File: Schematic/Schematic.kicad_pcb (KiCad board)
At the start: 2 copper layers, 67.5 x 55 mm, 17 parts, among them J3 FTDI, SW1 SW_Push, U1 ATmega328P-A, Y1 16 Mhz

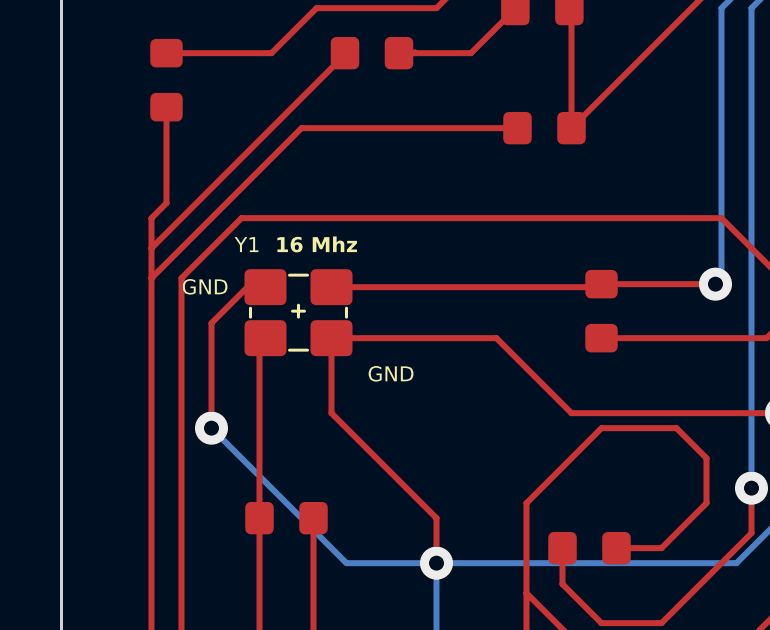
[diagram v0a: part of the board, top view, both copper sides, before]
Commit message: warnings still to do
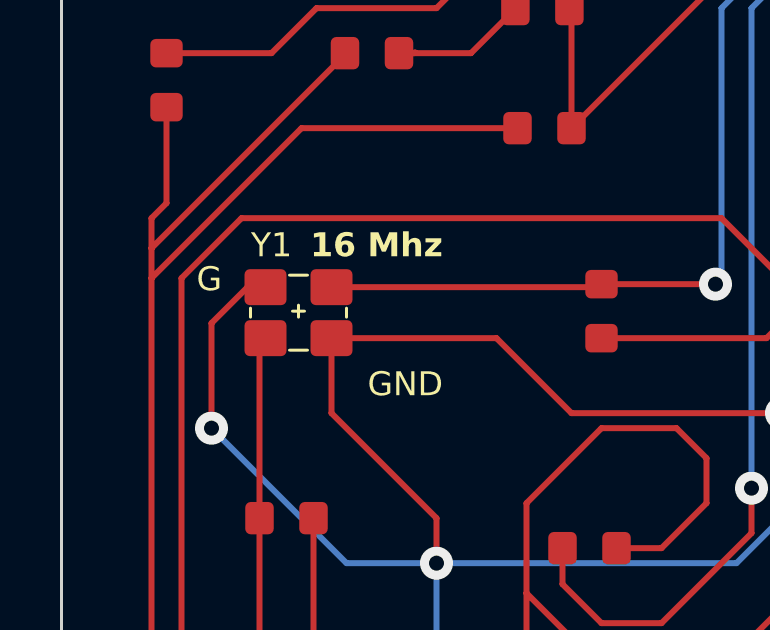
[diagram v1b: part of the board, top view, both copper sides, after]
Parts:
- C1, C2, C3, C4, C6, C7, D1, D2, R1, R2, R3: footprint Library:SMD_603 -> Library:SmD_603
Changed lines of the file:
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@@
 	(net 32 "A7")
 	(net 33 "A4")
-	(footprint "Library:SMD_603"
+	(footprint "Library:SmD_603"
 		(layer "F.Cu")
 		(at 146.6 122.5)
@@
 		(embedded_fonts no)
 	)
-	(footprint "Library:SMD_603"
+	(footprint "Library:SmD_603"
 		(layer "F.Cu")
 		(at 136.5 121.5)
@@
 			)
 		)
-		(property "Datasheet" "https://yageogroup.com/content/datasheet/asset/file/UPY-GPHC_X7R_6_3V-TO-250V"
+		(property "Datasheet" "https://yageogroup.com/content/datasheet/asset/file/PYU-RC_GROUP_51_ROHS_L"
 			(at 0 0 0)
 			(unlocked yes)
@@
 			(at -0.9 0)
 			(size 0.95 1.08)
-			(layers "F.Cu" "F.Paste")
+			(layers "F.Cu")
 			(roundrect_rratio 0.1968503937)
 			(net 3 "Net-(U1-XTAL1{slash}PB6)")
@@
 			(at 0.9 0)
 			(size 0.95 1.08)
-			(layers "F.Cu" "F.Paste")
+			(layers "F.Cu")
 			(roundrect_rratio 0.1968503937)
 			(net 2 "Net-(#PWR8-Pad1)")
@@
 		(embedded_fonts no)
 	)
-	(footprint "Library:SMD_603"
+	(footprint "Library:SmD_603"
 		(layer "F.Cu")
 		(at 145.1 108.5 180)
@@
 			)
 		)
-		(property "Datasheet" "https://yageogroup.com/content/datasheet/asset/file/UPY-GPHC_X7R_6_3V-TO-250V"
+		(property "Datasheet" "https://yageogroup.com/content/datasheet/asset/file/PYU-RC_GROUP_51_ROHS_L"
 			(at 0 0 180)
 			(unlocked yes)
@@
 			(at -0.9 0 180)
 			(size 0.95 1.08)
-			(layers "F.Cu" "F.Paste")
+			(layers "F.Cu")
 			(roundrect_rratio 0.1968503937)
 			(net 6 "RAW")
@@
 			(at 0.9 0 180)
 			(size 0.95 1.08)
-			(layers "F.Cu" "F.Paste")
+			(layers "F.Cu")
 			(roundrect_rratio 0.1968503937)
 			(net 17 "GND")
 			(pintype "passive")
+			(teardrops
+				(best_length_ratio 0.5)
+				(max_length 1)
+				(best_width_ratio 1)
+				(max_width 2)
+				(curved_edges no)
+				(filter_ratio 0.9)
+				(enabled yes)
+				(allow_two_segments yes)
+				(prefer_zone_connections yes)
+			)
 		)
 		(embedded_fonts no)
@@
 		(embedded_fonts no)
 	)
-	(footprint "Library:SMD_603"
+	(footprint "Library:SmD_603"
 		(layer "F.Cu")
 		(at 168.5 116.6 -90)
@@
 			)
 		)
-		(property "Datasheet" "https://yageogroup.com/content/datasheet/asset/file/UPY-GPHC_X7R_6_3V-TO-250V"
+		(property "Datasheet" "https://yageogroup.com/content/datasheet/asset/file/PYU-RC_GROUP_51_ROHS_L"
 			(at 0 0 270)
 			(unlocked yes)
@@
 			(at -0.9 0 270)
 			(size 0.95 1.08)
-			(layers "F.Cu" "F.Paste")
+			(layers "F.Cu")
 			(roundrect_rratio 0.1968503937)
 			(net 24 "VCC")
@@
 			(at 0.9 0 270)
 			(size 0.95 1.08)
-			(layers "F.Cu" "F.Paste")
+			(layers "F.Cu")
 			(roundrect_rratio 0.1968503937)
 			(net 4 "Net-(U1-AREF)")
@@
 		(embedded_fonts no)
 	)
-	(footprint "Library:SMD_603"
+	(footprint "Library:SmD_603"
 		(layer "F.Cu")
 		(at 163 116.6 -90)
@@
 		(embedded_fonts no)
 	)
-	(footprint "Library:SMD_603"
+	(footprint "Library:SmD_603"
 		(layer "F.Cu")
 		(at 147 139.5 90)
@@
 			)
 		)
-		(property "Datasheet" "https://yageogroup.com/content/datasheet/asset/file/UPY-GPHC_X7R_6_3V-TO-250V"
+		(property "Datasheet" "https://yageogroup.com/content/datasheet/asset/file/PYU-RC_GROUP_51_ROHS_L"
 			(at 0 0 90)
 			(unlocked yes)
@@
 		(embedded_fonts no)
 	)
-	(footprint "Library:SMD_603"
+	(footprint "Library:SmD_603"
 		(layer "F.Cu")
 		(at 132.5 106.9 -90)
@@
 			)
 		)
-		(property "Datasheet" "https://yageogroup.com/content/datasheet/asset/file/UPY-GPHC_X7R_6_3V-TO-250V"
+		(property "Datasheet" "https://yageogroup.com/content/datasheet/asset/file/PYU-RC_GROUP_51_ROHS_L"
 			(at 0 0 270)
 			(unlocked yes)
@@
 			(at -0.9 0 270)
 			(size 0.95 1.08)
-			(layers "F.Cu" "F.Paste")
+			(layers "F.Cu")
 			(roundrect_rratio 0.1968503937)
 			(net 6 "RAW")
@@
 			(at 0.9 0 270)
 			(size 0.95 1.08)
-			(layers "F.Cu" "F.Paste")
+			(layers "F.Cu")
 			(roundrect_rratio 0.1968503937)
 			(net 17 "GND")
@@
 		(embedded_fonts no)
 	)
-	(footprint "Library:SMD_603"
+	(footprint "Library:SmD_603"
 		(layer "F.Cu")
 		(at 147 114.6 -90)
@@
 			)
 		)
-		(property "Datasheet" "https://yageogroup.com/content/datasheet/asset/file/UPY-GPHC_X7R_6_3V-TO-250V"
+		(property "Datasheet" "https://yageogroup.com/content/datasheet/asset/file/PYU-RC_GROUP_51_ROHS_L"
 			(at 0 0 270)
 			(unlocked yes)
@@
 			(at -0.9 0 270)
 			(size 0.95 1.08)
-			(layers "F.Cu" "F.Paste")
+			(layers "F.Cu")
 			(roundrect_rratio 0.1968503937)
 			(net 1 "Net-(U1-XTAL2{slash}PB7)")
@@
 			(at 0.9 0 270)
 			(size 0.95 1.08)
-			(layers "F.Cu" "F.Paste")
+			(layers "F.Cu")
 			(roundrect_rratio 0.1968503937)
 			(net 2 "Net-(#PWR8-Pad1)")
@@
 		(embedded_fonts no)
 	)
-	(footprint "Library:SMD_603"
+	(footprint "Library:SmD_603"
 		(layer "F.Cu")
 		(at 158 116.5 90)
@@
 			)
 		)
-		(property "Datasheet" "https://cdn-reichelt.de/documents/datenblatt/A500/KP-1608ID(VER.9A).pdf"
+		(property "Datasheet" "https://yageogroup.com/content/datasheet/asset/file/PYU-RC_GROUP_51_ROHS_L"
 			(at 0 0 90)
 			(unlocked yes)
@@
 		(embedded_fonts no)
 	)
-	(footprint "Library:SMD_603"
+	(footprint "Library:SmD_603"
 		(layer "F.Cu")
 		(at 145.03 104.53 180)
@@
 			)
 		)
-		(property "Datasheet" "https://cdn-reichelt.de/documents/datenblatt/A500/KP-1608ID(VER.9A).pdf"
+		(property "Datasheet" "https://yageogroup.com/content/datasheet/asset/file/PYU-RC_GROUP_51_ROHS_L"
 			(at 0 0 180)
 			(unlocked yes)
@@
 		(at 136.9 114.6)
 		(property "Reference" "Y1"
-			(at -1.7 -2.2 0)
+			(at -0.9 -2.2 0)
 			(unlocked yes)
 			(layer "F.SilkS")
 			(effects
 				(font
-					(size 0.5 0.5)
+					(size 0.8 0.8)
 					(thickness 0.1)
 				)
@@
 		)
 		(property "Value" "16 Mhz"
-			(at 0.6 -2.2 0)
+			(at 2.6 -2.2 0)
 			(unlocked yes)
 			(layer "F.SilkS")
 			(effects
 				(font
-					(size 0.5 0.5)
+					(size 0.8 0.8)
 					(thickness 0.1)
 					(bold yes)
@@
 			(layer "F.CrtYd")
 		)
-		(fp_text user "GND"
-			(at -3.9 -0.5 0)
+		(fp_text user "G"
+			(at -3.4 -0.6 0)
 			(unlocked yes)
 			(layer "F.SilkS")
 			(effects
 				(font
-					(size 0.5 0.5)
+					(size 0.8 0.8)
 					(thickness 0.1)
 				)
@@
 		)
 		(fp_text user "GND"
-			(at 2.3 2.4 0)
+			(at 2.3 2.9 0)
 			(unlocked yes)
 			(layer "F.SilkS")
 			(effects
 				(font
-					(size 0.5 0.5)
+					(size 0.8 0.8)
 					(thickness 0.1)
 				)
@@
 		(embedded_fonts no)
 	)
-	(footprint "Library:SMD_603"
+	(footprint "Library:SmD_603"
 		(layer "F.Cu")
 		(at 139.35 106 180)
@@
 		(net 29)
 	)
+	(zone
+		(net 17)
+		(net_name "GND")
+		(layer "F.Cu")
+		(name "$teardrop_padvia$")
+		(hatch none 0.1)
+		(priority 30000)
+		(attr
+			(teardrop
+				(type padvia)
+			)
+		)
+		(connect_pads yes
+			(clearance 0)
+		)
+		(min_thickness 0.0254)
+		(filled_areas_thickness no)
+		(fill yes
+			(thermal_gap 0.5)
+			(thermal_bridge_width 0.5)
+			(island_removal_mode 1)
+			(island_area_min 10)
+		)
+		(polygon
+			(pts
+				(xy 143.25 108.4) (xy 143.25 108.6) (xy 143.77294 108.975) (xy 144.201 108.5) (xy 143.77294 108.025)
+			)
+		)
+	)
 	(embedded_fonts no)
